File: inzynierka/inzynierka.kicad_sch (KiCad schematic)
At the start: 32 parts, among them J101 Conn_01x10, U101 LM1117-3.3, U102 MCP6L04x-xSL, U103 LM239D

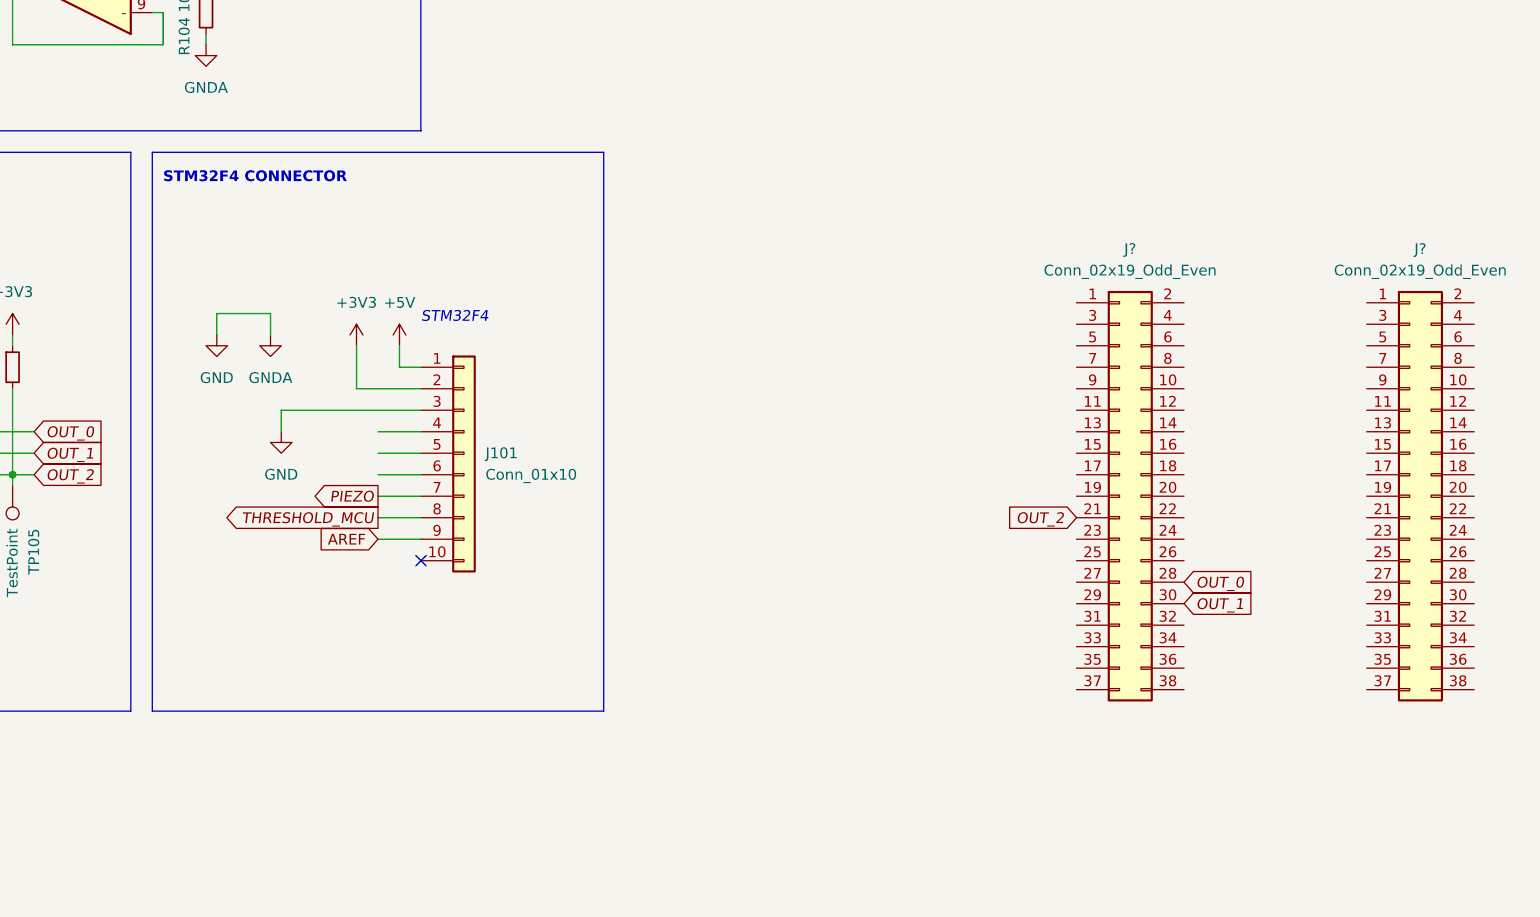
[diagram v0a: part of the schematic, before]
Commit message: shield shape
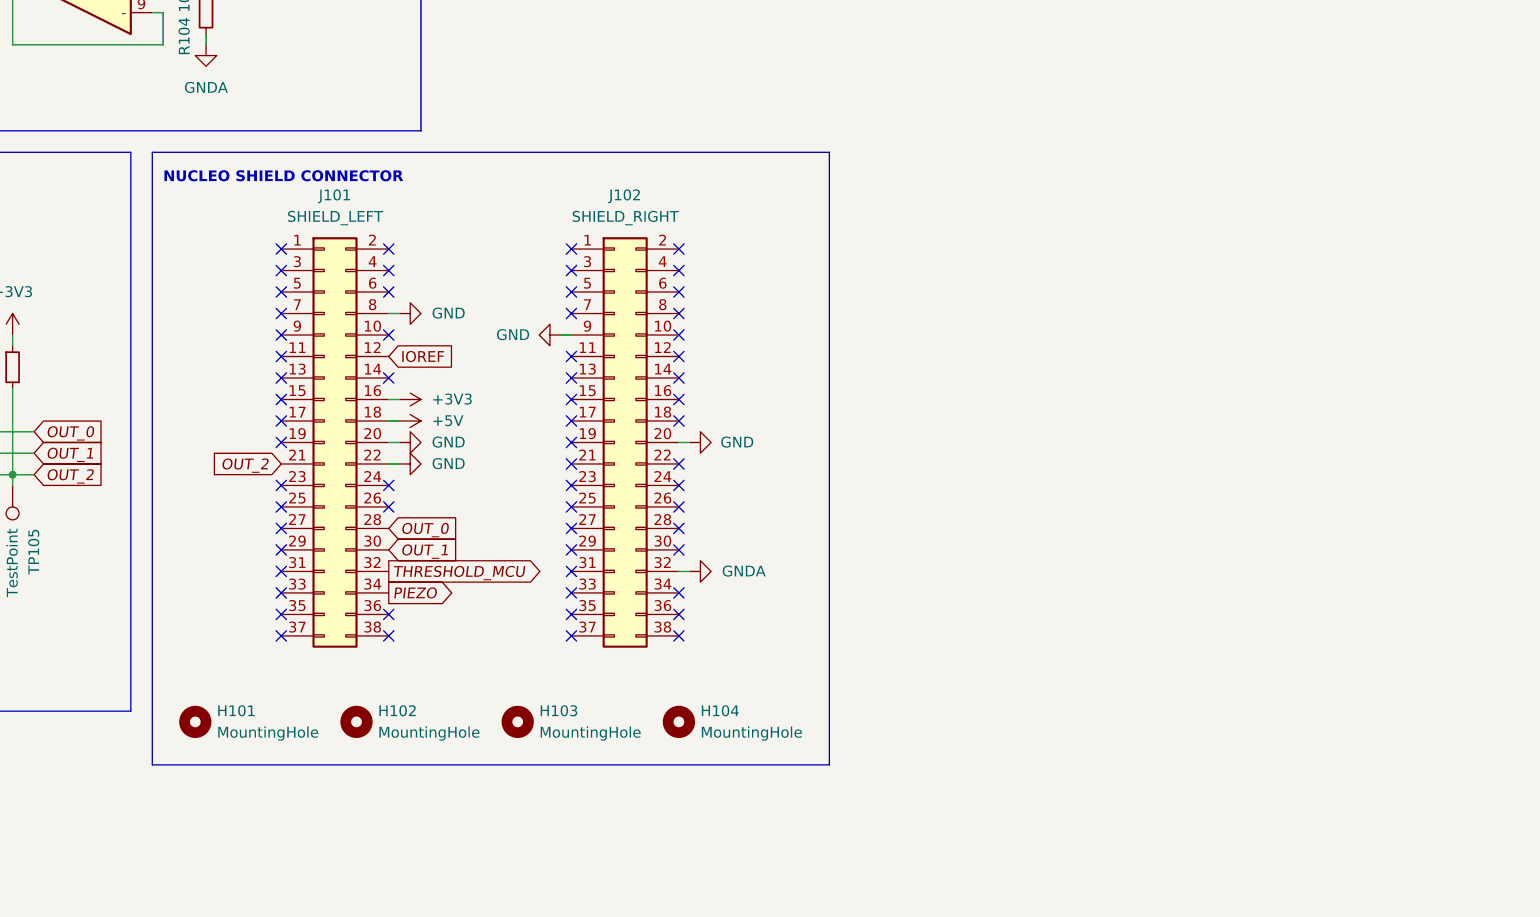
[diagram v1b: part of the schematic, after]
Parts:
- removed J101: Conn_01x10, Connector_JST:JST_XH_B10B-XH-A_1x10_P2.50mm_Vertical, symbol Connector_Generic:Conn_01x10
- added H101, H102, H103, H104: MountingHole, MountingHole:MountingHole_3.2mm_M3, symbol Mechanical:MountingHole
- J101: renamed from J?; value Conn_02x19_Odd_Even -> SHIELD_LEFT; footprint (none) -> Connector_PinSocket_2.54mm:PinSocket_2x19_P2.54mm_Vertical
- J102: renamed from J?; value Conn_02x19_Odd_Even -> SHIELD_RIGHT; footprint (none) -> Connector_PinSocket_2.54mm:PinSocket_2x19_P2.54mm_Vertical
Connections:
- net +3V3: now also J101.16 (Pin_16)
- net +5V: now also J101.18 (Pin_18)
- net GND: now also J101.20 (Pin_20), J101.22 (Pin_22), J101.8 (Pin_8), J102.20 (Pin_20), J102.9 (Pin_9); no longer C105.2, C107.2, C108.2, R104.2, R106.2, U102.11 (V-)
- net PIEZO: now also J101.34 (Pin_34)
- net THRESHOLD_MCU: now also J101.32 (Pin_32)
- net GNDA: now reaches J102.32 (Pin_32)
- net GNDA: now also C105.2, C107.2, C108.2, R104.2, R106.2, U102.11 (V-)
- net IOREF: now reaches J101.12 (Pin_12)
- no-connect marks 3 -> 64
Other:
- note added: "NUCLEO SHIELD CONNECTOR"
- note removed: "STM32F4"
- note removed: "STM32F4 CONNECTOR"
- moved on the sheet: J101, J102

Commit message: skonczone pcb
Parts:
- added BZ101: Buzzer, Buzzer_Beeper:Buzzer_15x7.5RM7.6, symbol Device:Buzzer
- added C112, C201, C301, C401: 100n, Capacitor_SMD:C_0603_1608Metric, symbol Device:C_Small
- added D104: DBG, LED_SMD:LED_0603_1608Metric, symbol Device:LED_Small
- added H105: BuzzerHole, MountingHole:MountingHole_2.2mm_M2, symbol Mechanical:MountingHole
- added J104: PIEZO, Connector_PinHeader_2.54mm:PinHeader_1x02_P2.54mm_Vertical, symbol Connector_Generic:Conn_01x02
- added J105, J106: FPC, Connector_FFC-FPC:Hirose_FH12-10S-0.5SH_1x10-1MP_P0.50mm_Horizontal, symbol Connector_Generic:Conn_01x10
- added R110, R111: 1k, Resistor_SMD:R_0603_1608Metric, symbol Device:R_Small
- added R112: 10k, Resistor_SMD:R_0603_1608Metric, symbol Device:R_Small
- added SW101: DBG, Button_Switch_SMD:SW_SPST_B3S-1000, symbol Switch:SW_DPST_x2
- added TP107: B+, TestPoint:TestPoint_Pad_D2.0mm, symbol Connector:TestPoint
- added TP108: B-, TestPoint:TestPoint_Pad_D2.0mm, symbol Connector:TestPoint
- added U201, U301, U401: SPU0410LR5H-QB, SPU0410:SPU0410LR5H-QB, symbol SPU0410LR5H-QB:SPU0410LR5H-QB
- TP101, TP106: value TestPoint -> THR
- TP102: value TestPoint -> OP
- TP103: value TestPoint -> OUT_0
- TP104: value TestPoint -> OUT_1
- TP105: value TestPoint -> OUT_2
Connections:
- net +3V3: now also C201.1, C301.1, C401.1, J105.10 (Pin_10), J105.9 (Pin_9), J106.1 (Pin_1), J106.2 (Pin_2), R110.1, R112.1, U201.4 (VDD), U301.4 (VDD), U401.4 (VDD)
- net GND: now also C105.2, C107.2, C108.2, R104.2, R106.2, U102.11 (V-), C112.2, C201.2, C301.2, C401.2, J105.1 (Pin_1), J105.2 (Pin_2), J105.4 (Pin_4), J105.6 (Pin_6), J105.8 (Pin_8), J106.10 (Pin_10), J106.3 (Pin_3), J106.5 (Pin_5), J106.7 (Pin_7), J106.9 (Pin_9), SW101.2 (B), U201.2 (GND), U201.3 (GND), U201.5 (GND), U201.6 (GND), U301.2 (GND), U301.3 (GND), U301.5 (GND), U301.6 (GND), U401.2 (GND), U401.3 (GND), U401.5 (GND), U401.6 (GND)
- net GNDA: no longer C105.2, C107.2, C108.2, R104.2, R106.2, U102.11 (V-)
- net PIEZO: now also J102.13 (Pin_13); no longer J101.34 (Pin_34)
- net DBG_LED: now reaches J102.1 (Pin_1)
- net DBG_LED: now also D104.2 (A)
- net DBG_BUT: now reaches J101.2 (Pin_2)
- net DBG_BUT: now also R111.2, R112.2
- new net: J105.3 (Pin_3), U301.1 (OUTPUT)
- new net: D104.1 (K), R110.2
- new net: BZ101.1 (-), TP107.1
- new net: BZ101.2 (+), TP108.1
- new net: J105.5 (Pin_5), U201.1 (OUTPUT)
- new net: J105.7 (Pin_7), U401.1 (OUTPUT)
- new net: C112.1, R111.1, SW101.1 (A)
- new net MIC_0/MIC_RAW: J106.4 (Pin_4)
- new net MIC_1/MIC_RAW: J106.6 (Pin_6)
- new net MIC_2/MIC_RAW: J106.8 (Pin_8)
- new net TRANSMITER/BUZZER+: J104.1 (Pin_1)
- new net TRANSMITER/BUZZER-: J104.2 (Pin_2)
- no-connect marks 64 -> 62
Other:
- sheet MIC_0 ports: added MIC, MIC_RAW; removed MIC_0
- sheet MIC_1 ports: added MIC, MIC_RAW; removed MIC_1
- sheet MIC_2 ports: added MIC, MIC_RAW; removed MIC_2
- sheet TRANSMITER ports: added BUZZER+, BUZZER-, INPUT; removed PIEZO
- note added: "DEBUG BUTTON"
- note added: "MOUNTING HOLES"
- company: (none) -> Krystian Mirek
- title: (none) -> UltraSoundSensor
- moved on the sheet: C105, C106, C107, C108, D101, D102, D103, H101, H102, H103, H104, J101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
